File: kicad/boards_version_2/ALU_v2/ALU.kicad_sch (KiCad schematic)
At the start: 59 parts

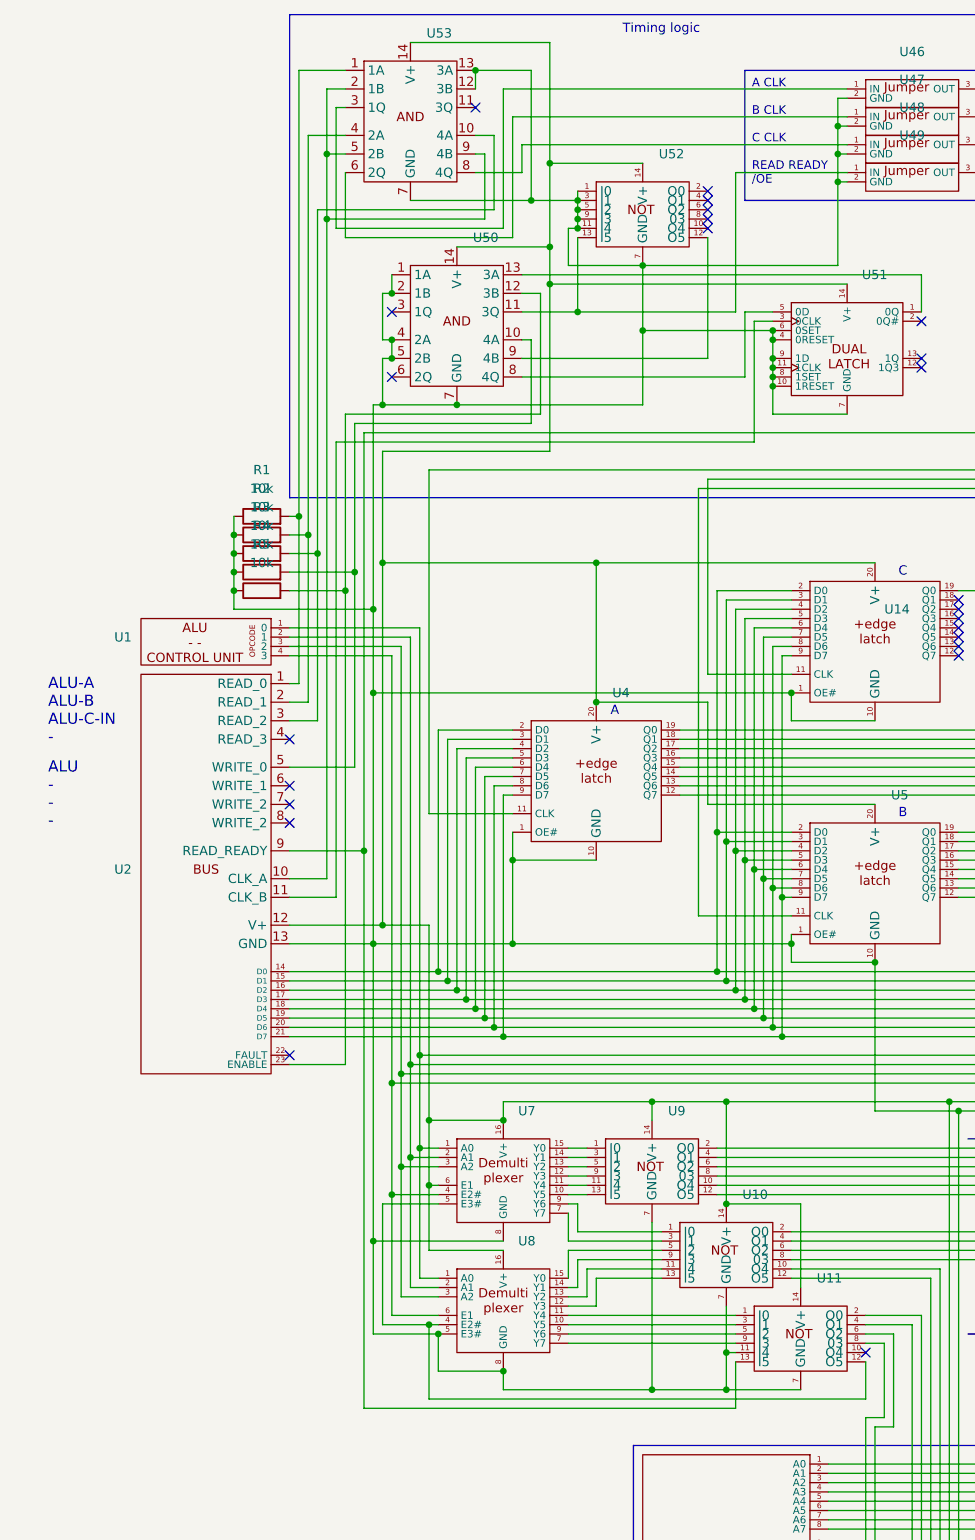
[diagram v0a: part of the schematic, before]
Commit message: Work mostly on bus
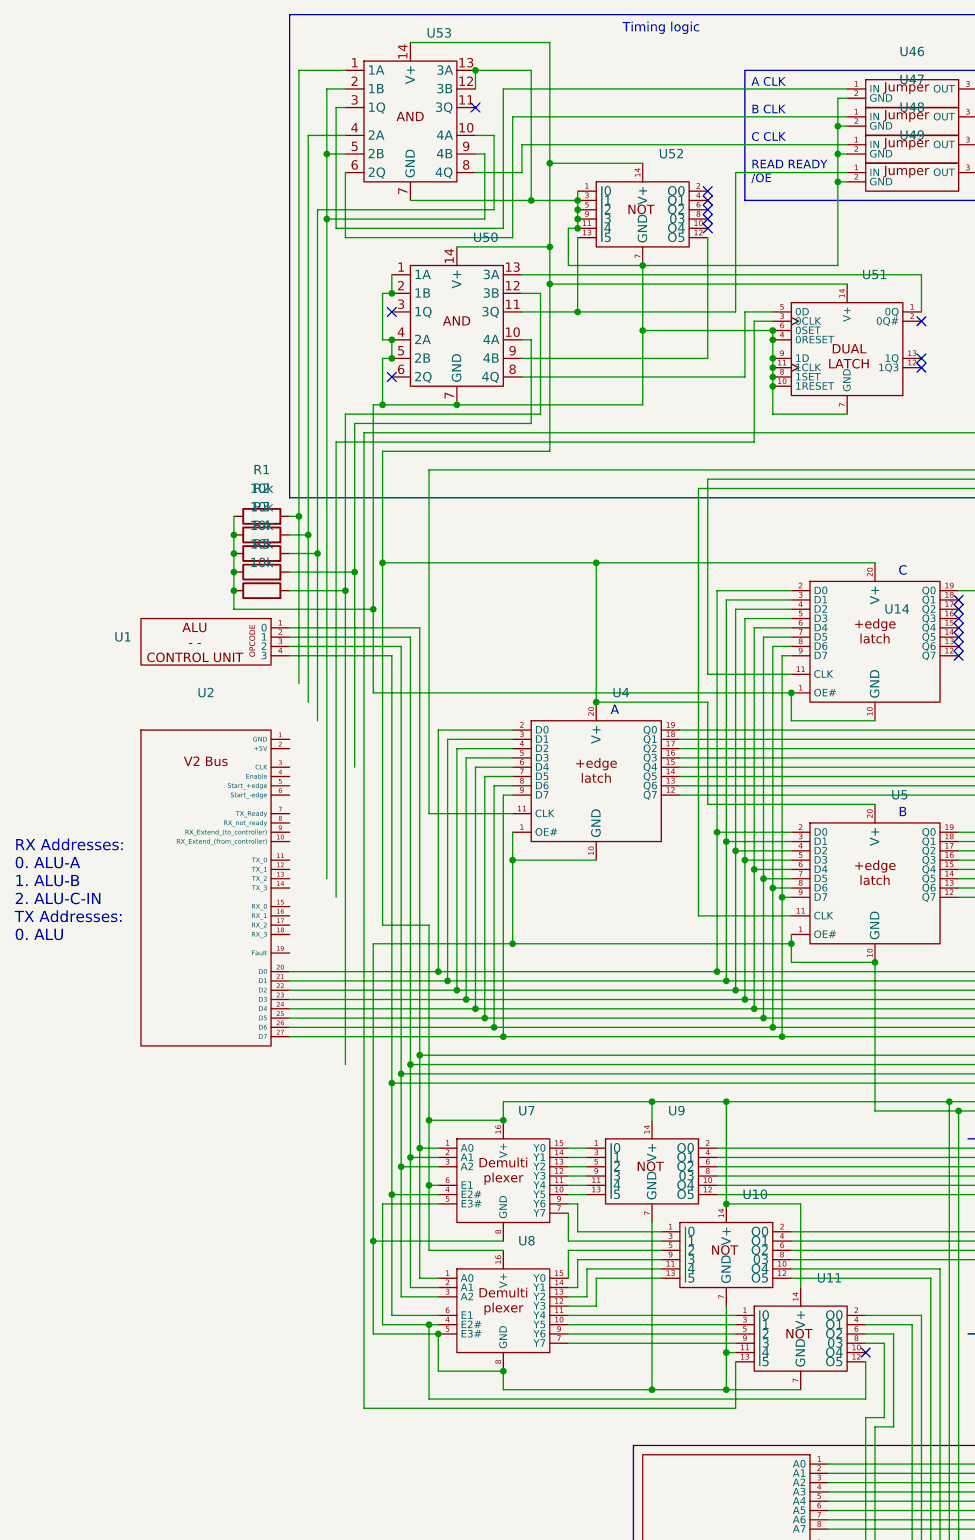
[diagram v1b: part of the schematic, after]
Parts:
- removed U2: ~, Connector_PinHeader_2.54mm:PinHeader_1x23_P2.54mm_Vertical, symbol custom_symbol_lib:bus_edge_connector
- added U2: ~, Connector_PinHeader_2.54mm:PinHeader_1x27_P2.54mm_Vertical, symbol custom_symbol_lib:bus_v2
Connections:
- net at U10.7 (GND), U11.11 (I4), U11.7 (GND)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: no longer R1.1, R2.1, R3.1, R4.1, R5.1, U14.1 (OE#), U14.10 (GND), U46.2 (GND), U47.2 (GND), U48.2 (GND), U49.2 (GND), U50.1 (1A), U50.2 (1B), U50.4 (2A), U50.5 (2B), U50.7 (GND), U51.10 (1RESET), U51.11 (1CLK), U51.4 (0RESET), U51.6 (0SET), U51.7 (GND), U51.8 (1SET), U51.9 (1D), U52.1 (I0), U52.11 (I4), U52.3 (I1), U52.5 (I2), U52.7 (GND), U52.9 (I3), U53.12 (3B), U53.13 (3A), U53.7 (GND)
- net at U14.9 (D7), U16.12 (Q7), U17.12 (Q7)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: now also U2.27 (D7)
- net at U14.8 (D6), U16.13 (Q6), U17.13 (Q6)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: now also U2.26 (D6)
- net at U14.7 (D5), U16.14 (Q5), U17.14 (Q5)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: now also U2.25 (D5)
- net at U14.6 (D4), U16.15 (Q4), U17.15 (Q4)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: now also U2.24 (D4)
- net at U14.5 (D3), U16.16 (Q3), U17.16 (Q3)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: now also U2.23 (D3)
- net at U14.4 (D2), U16.17 (Q2), U17.17 (Q2)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: now also U2.22 (D2)
- net at U14.3 (D1), U16.18 (Q1), U17.18 (Q1)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: now also U2.21 (D1)
- net at U14.2 (D0), U16.19 (Q0), U17.19 (Q0)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: now also U2.20 (D0)
- new net: R1.1, R2.1, R3.1, R4.1, R5.1, U14.1 (OE#), U14.10 (GND), U46.2 (GND), U47.2 (GND), U48.2 (GND), U49.2 (GND), U50.1 (1A), U50.2 (1B), U50.4 (2A), U50.5 (2B), U50.7 (GND), U51.10 (1RESET), U51.11 (1CLK), U51.4 (0RESET), U51.6 (0SET), U51.7 (GND), U51.8 (1SET), U51.9 (1D), U52.1 (I0), U52.11 (I4), U52.3 (I1), U52.5 (I2), U52.7 (GND), U52.9 (I3), U53.12 (3B), U53.13 (3A), U53.7 (GND)
- no-connect marks 42 -> 37
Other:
- note added: "RX Addresses: 0. ALU-A 1. ALU-B 2. ALU-C-IN TX Addresses: 0. ALU"
- note removed: "ALU - - -"
- note removed: "ALU-A ALU-B ALU-C-IN -"
